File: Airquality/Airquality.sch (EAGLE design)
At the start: 80 parts, among them IC1 SCD41-D-R2, U1 SGP41-D-R4, U3 BMP581, U4 AP22802AW5-7K-3.3V, U5 AP3602AKTR-G1

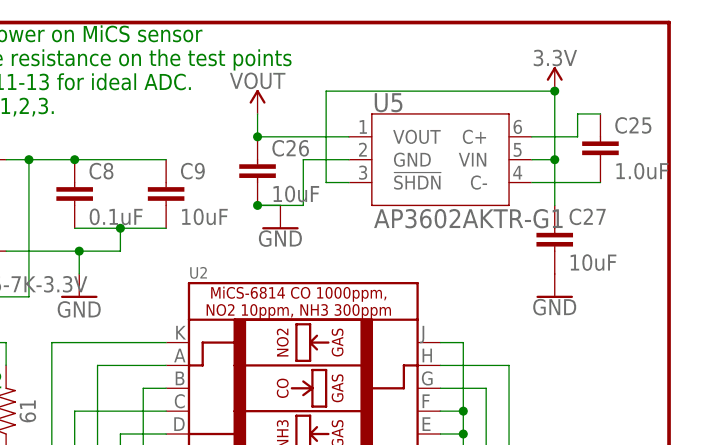
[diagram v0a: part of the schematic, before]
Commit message: Production Updates
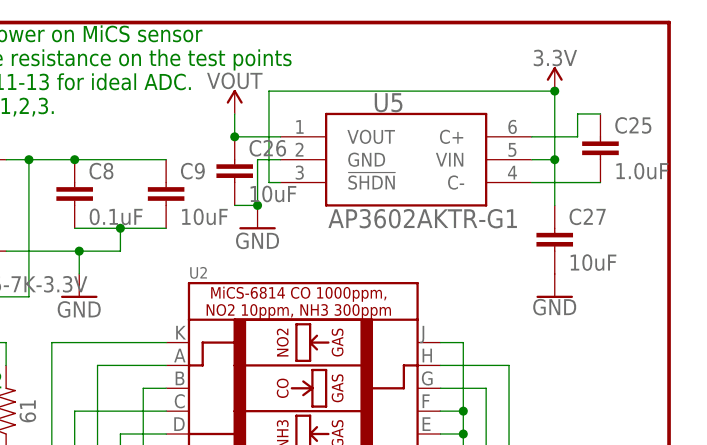
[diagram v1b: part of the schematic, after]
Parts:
- U5: device AP3602A:AP3602AKTR-G1 -> AP3602AKTR-G1:AP3602AKTR-G1
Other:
- moved on the sheet: C26
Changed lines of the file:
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@@
 <drawing>
 <settings>
-<setting alwaysvectorfont="no"/>
+<setting alwaysvectorfont="yes"/>
 <setting verticaltext="up"/>
 </settings>
@@
 <part name="C13" library="SparkFun-Capacitors" library_urn="urn:adsk.eagle:library:510" deviceset="0.1UF" device="-0402-16V-10%" package3d_urn="urn:adsk.eagle:package:37413/1" value="0.1uF"/>
 <part name="C24" library="SparkFun-Capacitors" library_urn="urn:adsk.eagle:library:510" deviceset="0.1UF" device="-0402-16V-10%" package3d_urn="urn:adsk.eagle:package:37413/1" value="0.1uF"/>
-<part name="U5" library="AP3602A" deviceset="AP3602AKTR-G1" device=""/>
+<part name="U5" library="AP3602AKTR-G1" deviceset="AP3602AKTR-G1" device=""/>
 <part name="SUPPLY4" library="SparkFun-PowerSymbols" library_urn="urn:adsk.eagle:library:530" deviceset="3.3V" device=""/>
 <part name="SUPPLY6" library="SparkFun-PowerSymbols" library_urn="urn:adsk.eagle:library:530" deviceset="3.3V" device=""/>
@@
 <attribute name="VALUE" x="116.586" y="-14.859" size="1.778" layer="96" font="vector"/>
 </instance>
-<instance part="U5" gate="A" x="81.28" y="73.66" smashed="yes">
+<instance part="U5" gate="G$1" x="81.28" y="73.66" smashed="yes">
 <attribute name="NAME" x="91.5416" y="76.4286" size="2.0828" layer="95" ratio="20" rot="SR0"/>
-<attribute name="VALUE" x="91.6686" y="63.5254" size="2.0828" layer="96" ratio="10" rot="SR0"/>
+<attribute name="VALUE" x="86.5886" y="63.5254" size="2.0828" layer="96" ratio="10" rot="SR0"/>
 </instance>
 <instance part="SUPPLY4" gate="G$1" x="20.32" y="76.2" smashed="yes">
@@
 <attribute name="VALUE" x="118.364" y="68.961" size="1.778" layer="96" font="vector"/>
 </instance>
-<instance part="C26" gate="G$1" x="78.74" y="68.58" smashed="yes">
-<attribute name="NAME" x="80.264" y="71.501" size="1.778" layer="95" font="vector"/>
-<attribute name="VALUE" x="80.264" y="66.421" size="1.778" layer="96" font="vector"/>
+<instance part="C26" gate="G$1" x="76.2" y="68.58" smashed="yes">
+<attribute name="NAME" x="77.724" y="71.501" size="1.778" layer="95" font="vector"/>
+<attribute name="VALUE" x="77.724" y="66.421" size="1.778" layer="96" font="vector"/>
 </instance>
 <instance part="C27" gate="G$1" x="111.76" y="60.96" smashed="yes">
@@
 <attribute name="VALUE" x="111.76" y="55.626" size="1.778" layer="96" align="top-center"/>
 </instance>
-<instance part="GND20" gate="1" x="81.28" y="63.5" smashed="yes">
-<attribute name="VALUE" x="81.28" y="63.246" size="1.778" layer="96" align="top-center"/>
-</instance>
-<instance part="SUPPLY7" gate="G$1" x="78.74" y="76.2" smashed="yes">
-<attribute name="VALUE" x="78.74" y="78.994" size="1.778" layer="96" align="bottom-center"/>
+<instance part="GND20" gate="1" x="78.74" y="63.5" smashed="yes">
+<attribute name="VALUE" x="78.74" y="62.992" size="1.778" layer="96" align="top-center"/>
+</instance>
+<instance part="SUPPLY7" gate="G$1" x="76.2" y="76.2" smashed="yes">
+<attribute name="VALUE" x="76.2" y="78.994" size="1.778" layer="96" align="bottom-center"/>
 </instance>
 <instance part="SUPPLY3" gate="G$1" x="-78.74" y="-48.26" smashed="yes">
@@
 <pinref part="C26" gate="G$1" pin="2"/>
 <pinref part="GND20" gate="1" pin="GND"/>
-<pinref part="U5" gate="A" pin="GND"/>
-<wire x1="88.9" y1="71.12" x2="83.82" y2="71.12" width="0.1524" layer="91"/>
-<wire x1="83.82" y1="71.12" x2="83.82" y2="66.04" width="0.1524" layer="91"/>
-<wire x1="83.82" y1="66.04" x2="78.74" y2="66.04" width="0.1524" layer="91"/>
+<pinref part="U5" gate="G$1" pin="GND"/>
+<wire x1="81.28" y1="71.12" x2="78.74" y2="71.12" width="0.1524" layer="91"/>
+<wire x1="78.74" y1="71.12" x2="78.74" y2="66.04" width="0.1524" layer="91"/>
 <junction x="78.74" y="66.04"/>
-<wire x1="78.74" y1="66.04" x2="81.28" y2="66.04" width="0.1524" layer="91"/>
+<wire x1="76.2" y1="66.04" x2="78.74" y2="66.04" width="0.1524" layer="91"/>
 </segment>
 </net>
@@
 </segment>
 <segment>
-<pinref part="U5" gate="A" pin="VIN"/>
+<pinref part="U5" gate="G$1" pin="VIN"/>
 <wire x1="109.22" y1="71.12" x2="111.76" y2="71.12" width="0.1524" layer="91"/>
 <pinref part="C27" gate="G$1" pin="1"/>
@@
 <junction x="111.76" y="71.12"/>
 <pinref part="SUPPLY2" gate="G$1" pin="3.3V"/>
-<pinref part="U5" gate="A" pin="!SHDN"/>
-<wire x1="88.9" y1="68.58" x2="86.36" y2="68.58" width="0.1524" layer="91"/>
-<wire x1="86.36" y1="68.58" x2="86.36" y2="78.74" width="0.1524" layer="91"/>
-<wire x1="86.36" y1="78.74" x2="111.76" y2="78.74" width="0.1524" layer="91"/>
+<pinref part="U5" gate="G$1" pin="!SHDN"/>
+<wire x1="81.28" y1="68.58" x2="80.01" y2="68.58" width="0.1524" layer="91"/>
+<wire x1="80.01" y1="68.58" x2="80.01" y2="78.74" width="0.1524" layer="91"/>
+<wire x1="80.01" y1="78.74" x2="111.76" y2="78.74" width="0.1524" layer="91"/>
 <junction x="111.76" y="78.74"/>
 </segment>
@@
 <net name="N$15" class="0">
 <segment>
-<pinref part="U5" gate="A" pin="C+"/>
+<pinref part="U5" gate="G$1" pin="C+"/>
 <wire x1="109.22" y1="73.66" x2="114.3" y2="73.66" width="0.1524" layer="91"/>
 <pinref part="C25" gate="G$1" pin="1"/>
@@
 <segment>
 <pinref part="C25" gate="G$1" pin="2"/>
-<pinref part="U5" gate="A" pin="C-"/>
+<pinref part="U5" gate="G$1" pin="C-"/>
 <wire x1="116.84" y1="68.58" x2="109.22" y2="68.58" width="0.1524" layer="91"/>
 </segment>
@@
 </segment>
 <segment>
-<pinref part="U5" gate="A" pin="VOUT"/>
+<pinref part="U5" gate="G$1" pin="VOUT"/>
 <pinref part="C26" gate="G$1" pin="1"/>
-<wire x1="88.9" y1="73.66" x2="78.74" y2="73.66" width="0.1524" layer="91"/>
+<wire x1="81.28" y1="73.66" x2="76.2" y2="73.66" width="0.1524" layer="91"/>
 <pinref part="SUPPLY7" gate="G$1" pin="VOUT"/>
-<wire x1="78.74" y1="73.66" x2="78.74" y2="76.2" width="0.1524" layer="91"/>
-<junction x="78.74" y="73.66"/>
-</segment>
-</net>
+<wire x1="76.2" y1="73.66" x2="76.2" y2="76.2" width="0.1524" layer="91"/>
+<junction x="76.2" y="73.66"/>
+</segment>
+</net>
